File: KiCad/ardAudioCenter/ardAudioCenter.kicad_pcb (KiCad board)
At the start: 2 copper layers, 99.7 x 66 mm, 27 parts, among them J1 2-pin_power_input_header, J3 4-pin_I2C_LCD_header, U1 2-pole_power_in_screw_terminal, U10 CD4052B, U11 MCP41010, U13 4-pole_RL-input_screw_terminal, U15 TEA5767_FM_Radio_Module, U16 VolR, U2 KY-040_Rotary_Encoder, U3 L7805, U5 KY-040_Rotary_Encoder, U6 JDY-62_Bluetooth_Module, U7 4-pole_RL-output_screw_termin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, U8 MCP41010, U9 VolL

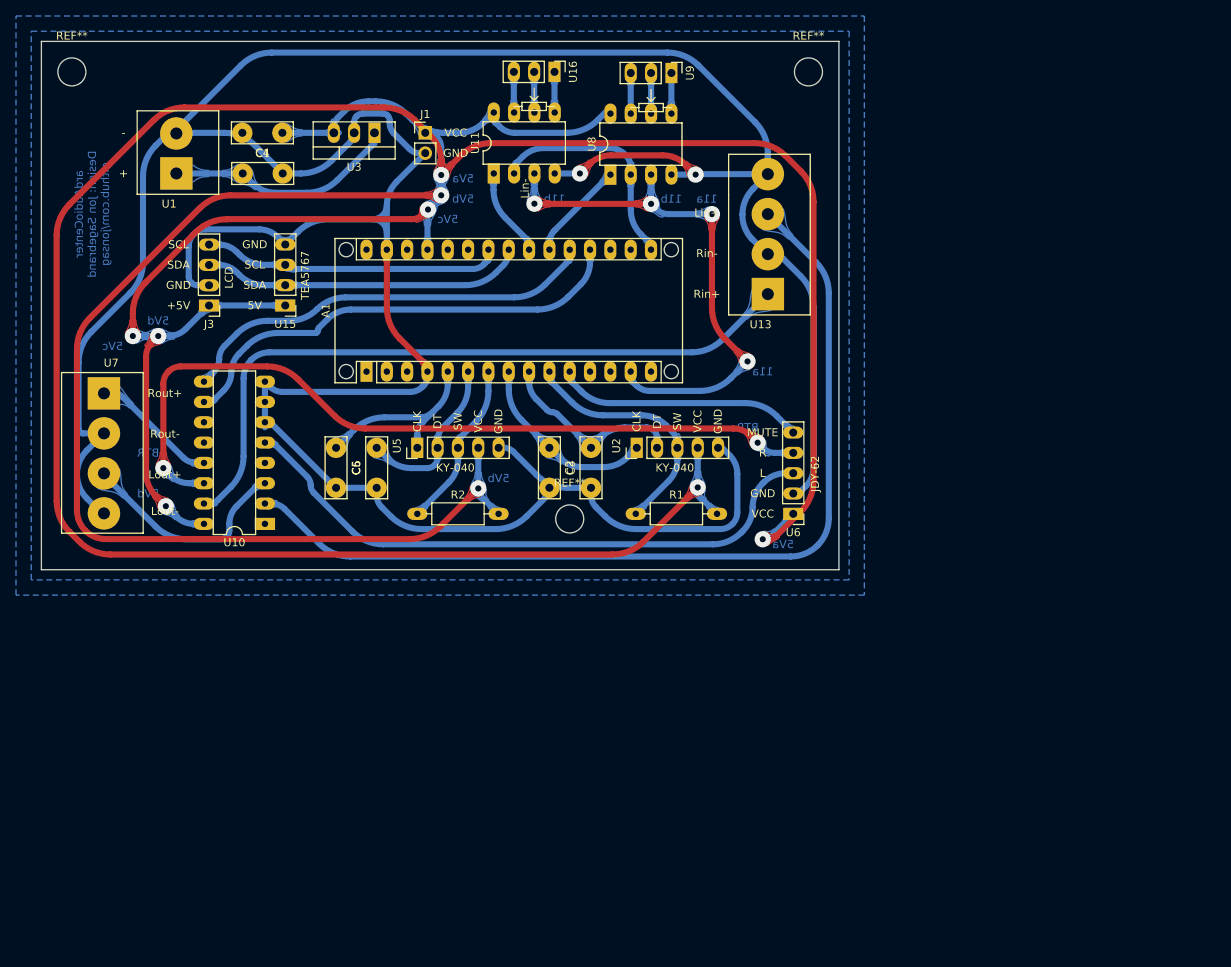
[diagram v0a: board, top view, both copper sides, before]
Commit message: PCBs
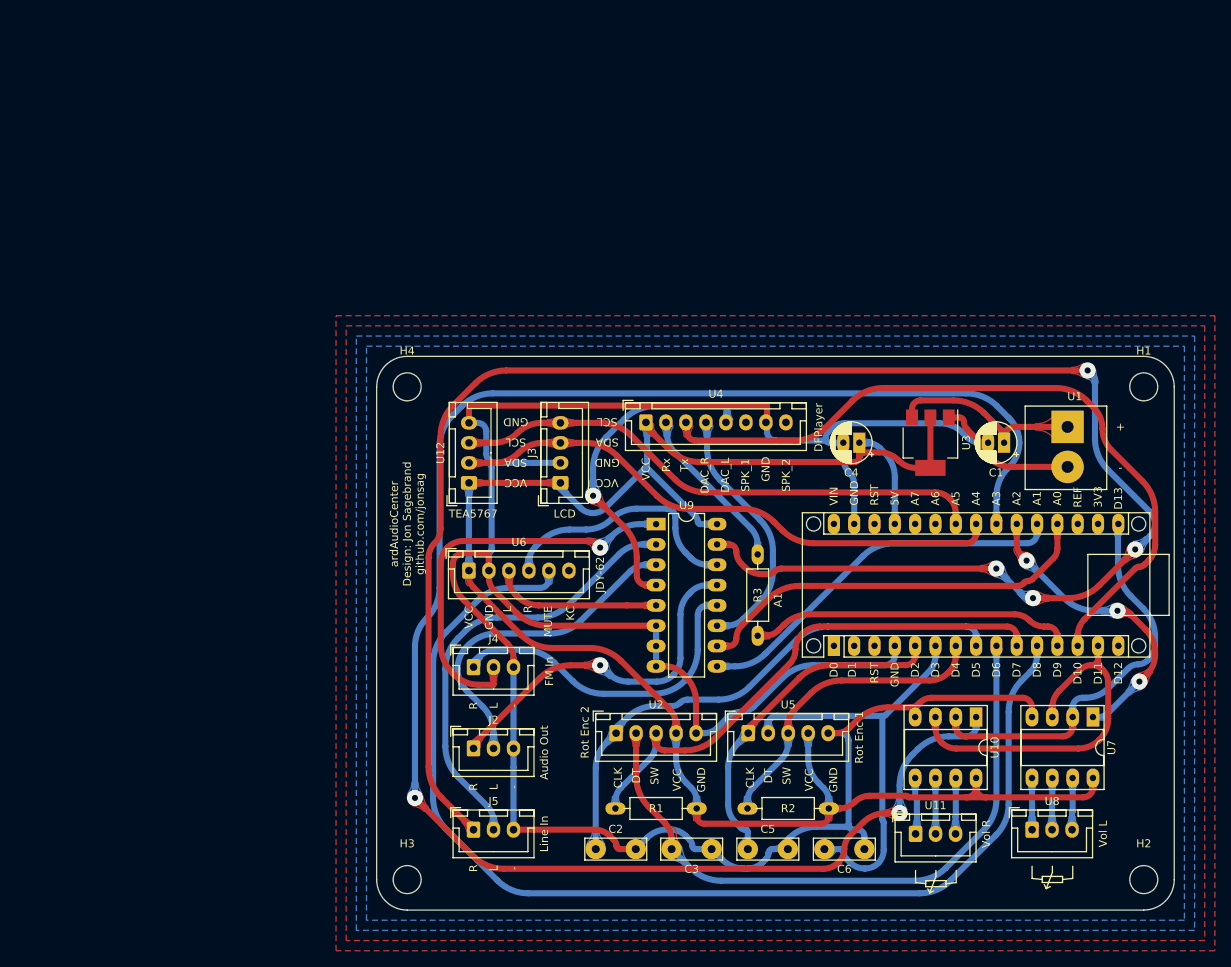
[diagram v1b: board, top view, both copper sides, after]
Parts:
- removed J1: 2-pin_power_input_header, My_Headers:2-pin_power_input_header
- removed REF** (x3): MountingHole_3.5mm, MountingHole:MountingHole_3.5mm
- removed U13: 4-pole_RL-input_screw_terminal, My_Parts:4-pole_screw_terminal_RL_input
- removed U15: TEA5767_FM_Radio_Module, My_Headers:4-pin_TEA5767_radio_module_header_large
- removed U16: VolR, My_Headers:3-pin_potentiometer_header_larger_pads
- added H1: MountingHole, MountingHole:MountingHole_3.5mm, F.Cu at (210.2, 80.0)
- added H2: MountingHole, MountingHole:MountingHole_3.5mm, F.Cu at (210.2, 141.6)
- added H3: MountingHole, MountingHole:MountingHole_3.5mm, F.Cu at (118.1, 141.6)
- added H4: MountingHole, MountingHole:MountingHole_3.5mm, F.Cu at (118.1, 80.0)
- added J2: Audio out, My_Headers:3-pin JST Audio, F.Cu at (126.4, 125.2)
- added J4: FM In, My_Headers:3-pin JST Audio, F.Cu at (126.4, 115.0)
- added J5: Line In, My_Headers:3-pin JST Audio, F.Cu at (126.4, 135.4)
- added R3: 330R, My_Misc:R_Axial_DIN0207_L6.3mm_D2.5mm_P10.16mm_Horizontal_larger_pads, F.Cu at (161.9, 101.0)
- added U12: FM Radio TEA5767, My_Headers:4-pin JST TEA5767 FM Radio, F.Cu at (125.8, 92.0)
- added U4: DFPlayer_Mini, My_Headers:8-pin JST DFPlayer Mini, F.Cu at (148.0, 84.5)
- C1: value 0.33u -> 10u; footprint My_Misc:C_Disc_D7.5mm_W2.5mm_P5.00mm_larger -> My_Misc:CP_Radial_D5.0mm_P2.00mm_larger
- C4: value 0.1u -> 22u; footprint My_Misc:C_Disc_D7.5mm_W2.5mm_P5.00mm_larger -> My_Misc:CP_Radial_D5.0mm_P2.00mm_larger
- J3: value 4-pin_I2C_LCD_header -> LCD; footprint My_Headers:4-pin_I2C_LCD_header_larger -> My_Headers:4-pin JST LCD
- U1: value 2-pole_power_in_screw_terminal -> Power In
- U10: value CD4052B -> MCP41010; footprint My_Misc:DIP-16_W7.62mm_larger -> My_Misc:DIP-8_W7.62mm_Socket_w_dip_packet_LongPads
- U11: value MCP41010 -> VolR; footprint My_Misc:DIP-8_W7.62mm_large -> My_Headers:3-pin JST Potentiometer
- U2: value KY-040_Rotary_Encoder -> Rotary encoder 2; footprint My_Headers:5-pin_KY-040_rotary_encoder_header_larger -> My_Headers:5-pin JST Rotary Encoder
- U3: value L7805 -> AMS1117-5.0; footprint My_Misc:TO-220-3_Vertical_larger -> Package_TO_SOT_SMD:SOT-223-3_TabPin2
- U5: value KY-040_Rotary_Encoder -> Rotary encoder 1; footprint My_Headers:5-pin_KY-040_rotary_encoder_header_larger -> My_Headers:5-pin JST Rotary Encoder
- U6: footprint My_Headers:5-pin_JDY-62_bluetooth_module_header_large -> My_Headers:6-pin JST JDY-62 Bluetooth
- U7: value 4-pole_RL-output_screw_terminal -> MCP41010; footprint My_Parts:4-pole_screw_terminal_RL_output -> My_Misc:DIP-8_W7.62mm_Socket_w_dip_packet_LongPads
- U8: value MCP41010 -> VolL; footprint My_Misc:DIP-8_W7.62mm_large -> My_Headers:3-pin JST Potentiometer
- U9: value VolL -> CD4052B; footprint My_Headers:3-pin_potentiometer_header_larger_pads -> My_Misc:DIP-16_W7.62mm_LongPads w socket
- moved U7 130.1 mm to (203.8, 121.3), turned to -90 degrees
- moved U1 115.8 mm to (200.7, 85.0), turned to 0 degrees
- moved C1 100.9 mm to (192.7, 87.0), turned to 180 degrees
- moved U11 98.0 mm to (181.7, 135.9), turned to 0 degrees
- moved U8 97.4 mm to (196.2, 135.4), turned to 0 degrees
- moved U10 92.1 mm to (189.2, 121.3), turned to -90 degrees
- moved C4 81.9 mm to (174.6, 87.0)
- moved U3 79.6 mm to (183.5, 87.0), turned to -90 degrees
- moved C6 75.9 mm to (175.3, 137.8), turned to 180 degrees
- moved C5 71.9 mm to (160.7, 137.8), turned to 0 degrees
- moved A1 67.7 mm to (171.4, 112.4)
- moved U9 56.4 mm to (149.2, 97.2), turned to 0 degrees
- moved R2 55.3 mm to (160.7, 132.7)
- moved U5 54.6 mm to (160.7, 123.3), turned to 0 degrees
- moved C2 50.5 mm to (141.7, 137.8), turned to 0 degrees
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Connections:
- J3 pad 3: GND -> /SDA
- U10 pad 1: FML+ -> /CSVolR
- U10 pad 2: LineL+ -> /SPI-SCK
- U10 pad 3: /Lout+ -> /SPI-COPI
- U10 pad 4: SDL+ -> GND
- U10 pad 5: BTL+ -> Net-(U10-Pad5)
- U10 pad 6: GND -> Net-(U10-Pad6)
- U10 pad 7: GND -> Net-(U10-Pad7)
- U10 pad 8: GND -> +5V
- U11 pad 1: /CSVolR -> Net-(U10-Pad5)
- U11 pad 2: /SPI-SCK -> Net-(U10-Pad6)
- U11 pad 3: /SPI-COPI -> Net-(U10-Pad7)
- U3 pad 1: +12V -> GND
- U3 pad 2: GND -> +5V
- U3 pad 3: +5V -> +12V
- U7 pad 1: /Rout+ -> /CSVolL
- U7 pad 2: GND -> /SPI-SCK
- U7 pad 3: /Lout+ -> /SPI-COPI
- U8 pad 1: /CSVolL -> Net-(U7-Pad5)
- U8 pad 2: /SPI-SCK -> Net-(U7-Pad6)
- U8 pad 3: /SPI-COPI -> Net-(U7-Pad7)
- U9 pad 1: Net-(U8-Pad5) -> Net-(J4-Pad2)
- U9 pad 2: Net-(U8-Pad6) -> Net-(J5-Pad2)
- U9 pad 3: Net-(U8-Pad7) -> /Lout+
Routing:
- net +5V: track 589.6 -> 230.8 mm, vias 9 -> 0
- net Net-(J5-Pad1): track 0.00 -> 221.2 mm, vias 0 -> 4
- net /CSVolR: track 11.1 -> 220.4 mm, vias 0 -> 2
- net LineL+: track 116.5 -> 0.00 mm
- net /BT-Mute: track 31.1 -> 141.7 mm
- net GND: track 447.0 -> 349.4 mm, vias 2 -> 0
- net /DFP-Tx: track 0.00 -> 91.8 mm
- net LineR+: track 88.2 -> 0.00 mm
- net BTR+: track 99.9 -> 31.7 mm, vias 2 -> 0
- net /RotEnc2-DT: track 24.1 -> 82.1 mm
- net BTL+: track 77.1 -> 21.2 mm
- net Net-(J5-Pad2): track 0.00 -> 55.3 mm
- net Net-(J4-Pad2): track 0.00 -> 51.5 mm, vias 0 -> 1
- net /RotEnc2-CLK: track 23.9 -> 67.1 mm
- net SDL+: track 0.00 -> 41.4 mm, vias 0 -> 1
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- added copper zone on F.Cu, net (none)
- added copper zone on F.Cu, net GND
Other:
- board size 99.7 x 66 mm -> 99.7 x 69.2 mm
- rule pad_to_mask_clearance: 0.05 -> 0
- board text added: "Audio Out"
- board text added: "Board size: 99,70 x 67,95"
- board text added: "DFPlayer"
- board text added: "FM In"
- board text added: "Hole CC: 92,08 x 61,60"
- board text added: "JDY-62"
- board text added: "LCD"
- board text added: "Line In"
- board text added: "Rot Enc 1"
- board text added: "Rot Enc 2"
- board text added: "TEA5767"
- board text added: "Vol L"
- board text added: "Vol R"
- board text removed: "11a"
- board text removed: "11b"
- board text removed: "5Va"
- board text removed: "5Vb"
- board text removed: "5Vc"
- board text removed: "5Vd"
- board text removed: "BTR"
